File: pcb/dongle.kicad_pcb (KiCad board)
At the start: 2 copper layers, 14 x 18.1 mm, 31 parts, among them J1 USB_A, J2 Conn_01x01_Pin, J3 Conn_01x01_Pin, J4 Conn_01x01_Pin, J5 Conn_01x01_Pin, SW1 SW_Push_45deg, U3 nRF52833_QDxx, Y1 Crystal_GND24, Y2 Crystal_Small

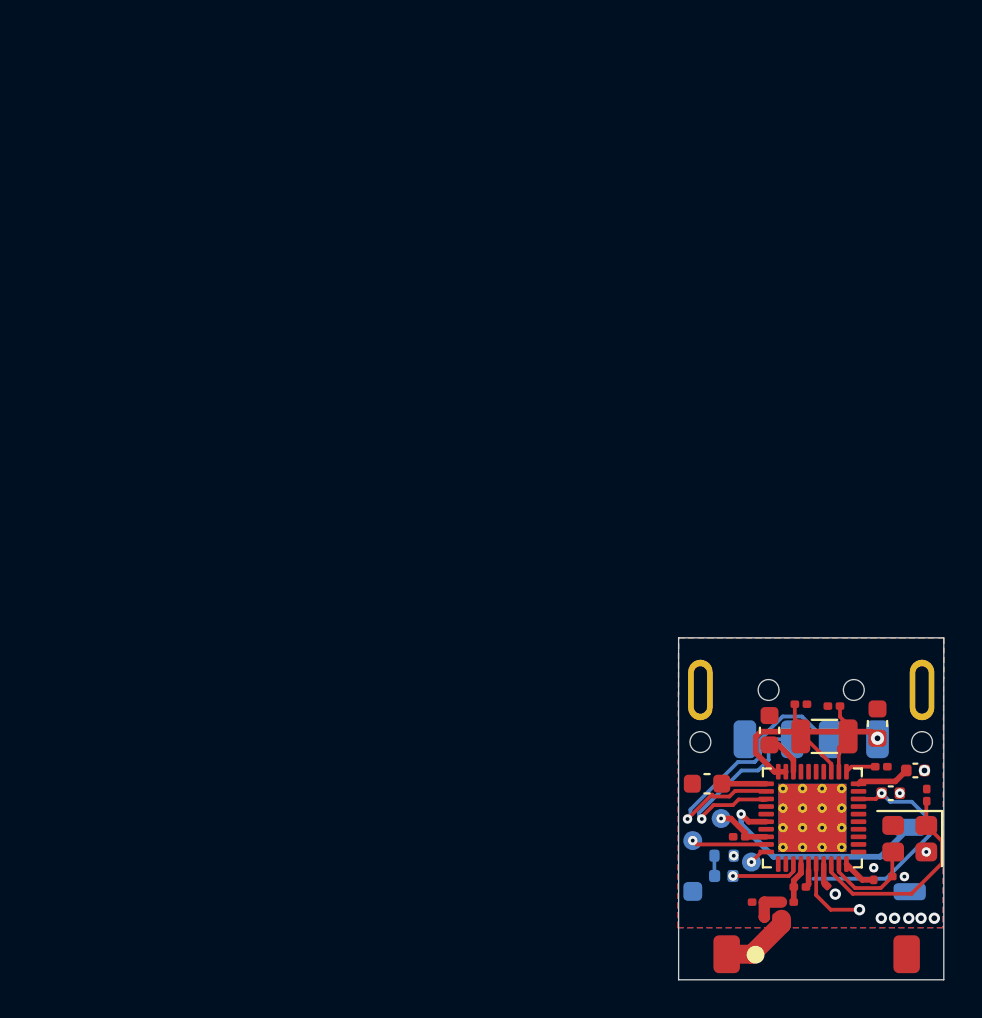
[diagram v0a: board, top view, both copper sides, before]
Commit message: update pcb
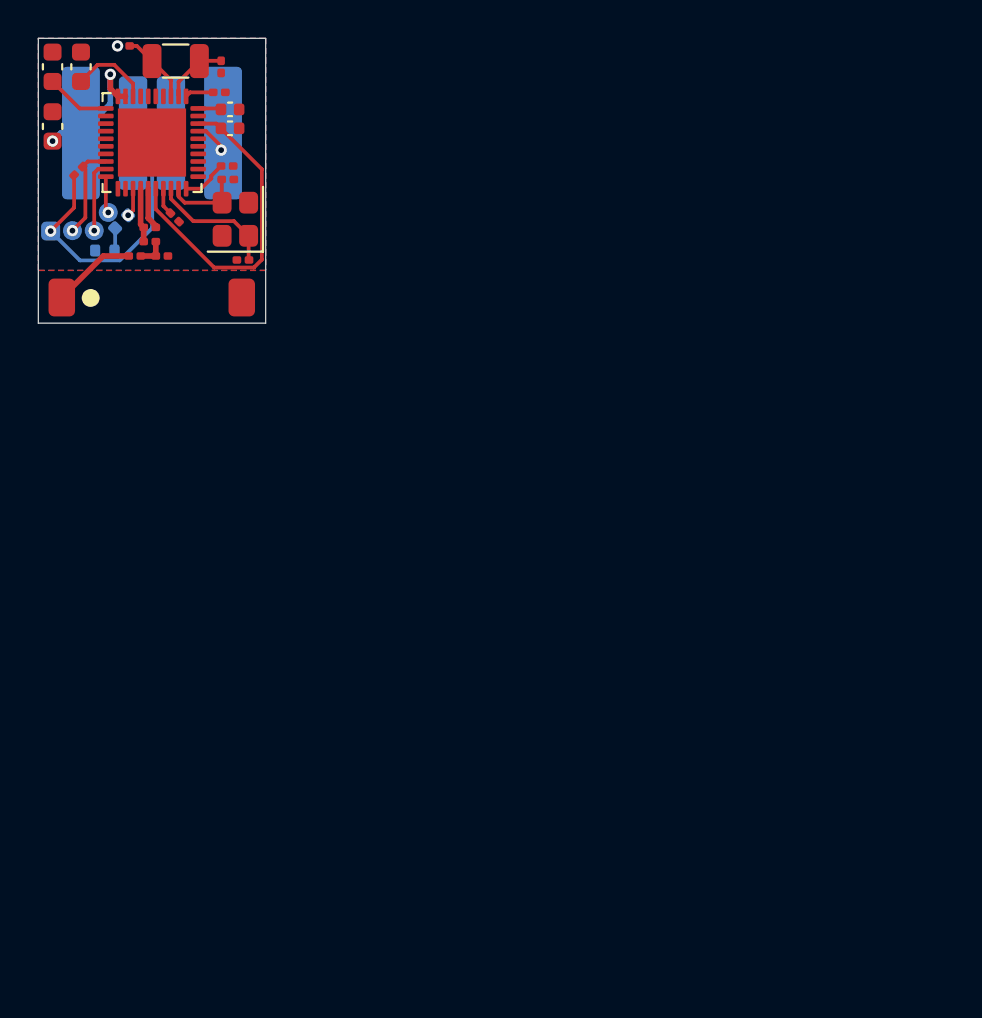
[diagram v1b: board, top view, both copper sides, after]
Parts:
- removed REF** (x2): MountingHole_1.1mm, dongle:MountingHole_1.1mm
- removed SW1: SW_Push_45deg, dongle:SW_SPST_B3U-1000P
- D1, R1: moved to F.Cu
- J1: footprint dongle:USB_A_Molex_48037-2200_Horizontal -> dongle:USB_A_PCB_Edge_receptacle
- U3: footprint dongle:QFN-40-1EP_5x5mm_P0.4mm_EP3.6x3.6mm_ThermalVias -> dongle:QFN-40-1EP_5x5mm_P0.4mm_EP3.6x3.6mm
- moved C17 53.8 mm to (142.9, 88.0)
- moved C19 51.2 mm to (142.9, 84.8), turned to -90 degrees
- moved C2 51.1 mm to (152.2, 90.8)
- moved C11 50.6 mm to (152.2, 90.1), turned to 180 degrees
- moved C6 50.5 mm to (144.4, 84.8)
- moved C12 50.3 mm to (152.3, 87.1)
- moved C5 49.9 mm to (151.8, 86.2)
- moved U3 49.9 mm to (148.2, 88.8)
- moved C15 49.9 mm to (146.7, 83.8), turned to 180 degrees
- moved C10 49.6 mm to (149.4, 92.8)
- moved C7 49.5 mm to (144.3, 90.3), turned to 45 degrees
- moved C13 49.5 mm to (152.3, 88.1)
- moved Y2 49.4 mm to (149.4, 84.5)
- moved AE1 49.3 mm to (146.3, 97.0)
- moved C3 48.9 mm to (148.1, 93.3)
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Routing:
- net GND: track 0.00 -> 16.4 mm, vias 12 -> 3
- net D-: track 15.9 -> 0.00 mm, vias 1 -> 0
- net RESET: track 12.3 -> 0.00 mm, vias 1 -> 0
- net D+: track 11.3 -> 0.00 mm, vias 1 -> 0
- net XC1: track 11.1 -> 6.73 mm
- net VDD: track 9.71 -> 12.9 mm
- net VBUS: track 9.59 -> 7.15 mm, vias 1 -> 2
- net LED: track 3.68 -> 1.52 mm
- net VSS_PA: track 0.95 -> 2.21 mm
- net XC2: track 5.16 -> 4.08 mm
- net DECUSB: track 2.35 -> 3.40 mm
- net SWC: track 1.00 -> 1.94 mm
- net ANT: track 2.17 -> 2.86 mm
- net DEC4_6: track 16.6 -> 17.3 mm, vias 2 -> 0
- net Net-(AE1-A): track 3.82 -> 4.44 mm
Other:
- board size 14 x 18.1 mm -> 12 x 15 mm
